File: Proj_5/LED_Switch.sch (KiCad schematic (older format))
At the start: 34 parts, among them SW1 SW_DIP_x08, U33 74LS374, U34 MAN72A, U36 74LS374, U37 MAN72A, U56 74LS374, U57 74LS244, U59 PAL16L8, U61 PAL16L8

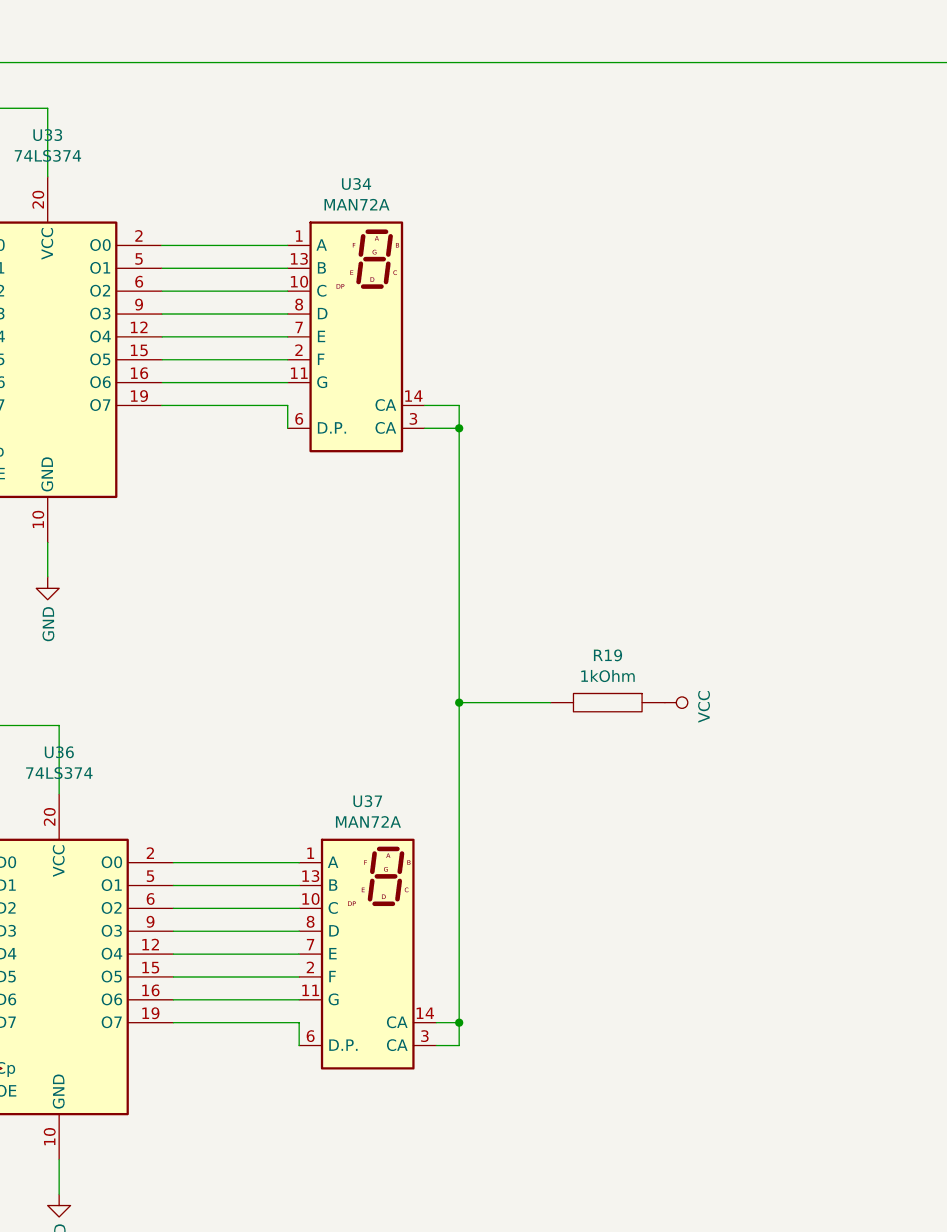
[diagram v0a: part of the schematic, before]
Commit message: Wires are Hell
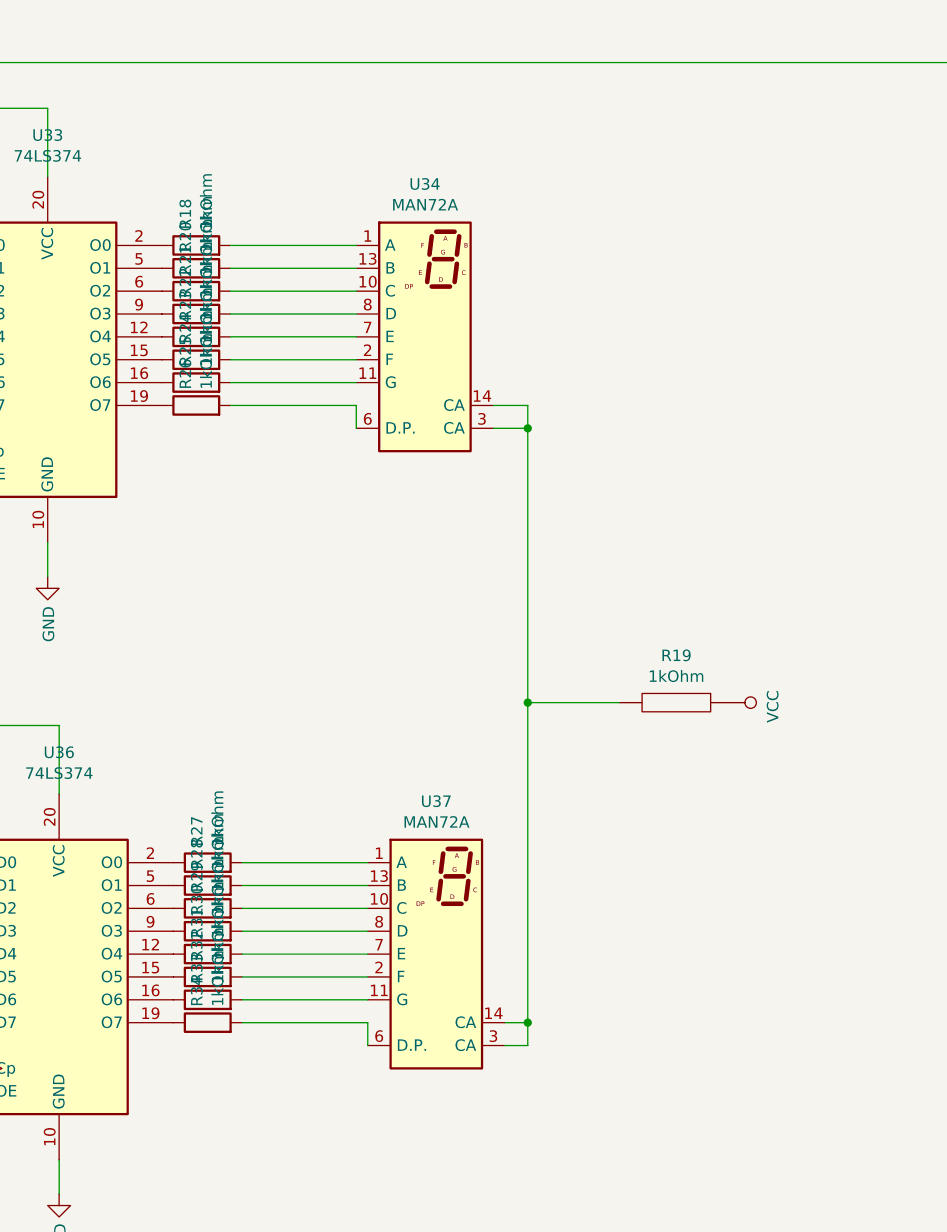
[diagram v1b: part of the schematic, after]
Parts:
- added R18, R20, R21, R22, R23, R24, R25, R26, R27, R28, R29, R30, R31, R32, R33, R34: 1kOhm, Resistor_SMD:R_1206_3216Metric, symbol Device:R
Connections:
- net at U37.1 (A): now also R27.2; no longer U36.2 (O0)
- net at U37.10 (C): now also R29.2; no longer U36.6 (O2)
- net at U37.11 (G): now also R33.2; no longer U36.16 (O6)
- net at U37.13 (B): now also R28.2; no longer U36.5 (O1)
- net at U37.2 (F): now also R32.2; no longer U36.15 (O5)
- net at U37.6 (D.P.): now also R34.2; no longer U36.19 (O7)
- net at U37.7 (E): now also R31.2; no longer U36.12 (O4)
- net at U37.8 (D): now also R30.2; no longer U36.9 (O3)
- net at U34.1 (A): now also R18.2; no longer U33.2 (O0)
- net at U34.10 (C): now also R21.2; no longer U33.6 (O2)
- net at U34.11 (G): now also R25.2; no longer U33.16 (O6)
- net at U34.13 (B): now also R20.2; no longer U33.5 (O1)
- net at U34.2 (F): now also R24.2; no longer U33.15 (O5)
- net at U34.6 (D.P.): now also R26.2; no longer U33.19 (O7)
- net at U34.7 (E): now also R23.2; no longer U33.12 (O4)
- net at U34.8 (D): now also R22.2; no longer U33.9 (O3)
- new net: R31.1, U36.12 (O4)
- new net: R32.1, U36.15 (O5)
- new net: R33.1, U36.16 (O6)
- new net: R34.1, U36.19 (O7)
- new net: R27.1, U36.2 (O0)
- new net: R28.1, U36.5 (O1)
- new net: R29.1, U36.6 (O2)
- new net: R30.1, U36.9 (O3)
- new net: R23.1, U33.12 (O4)
- new net: R24.1, U33.15 (O5)
- new net: R25.1, U33.16 (O6)
- new net: R26.1, U33.19 (O7)
- new net: R18.1, U33.2 (O0)
- new net: R20.1, U33.5 (O1)
- new net: R21.1, U33.6 (O2)
- new net: R22.1, U33.9 (O3)
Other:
- moved on the sheet: R19, U34, U37
